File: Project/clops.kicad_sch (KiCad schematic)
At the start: 111 parts, among them IC1 W25Q16JVUXIQ, J1 USB_C_Receptacle_USB2.0, SW1 boot, SW2 RotaryEncoder_Switch, U2 USBLC6-2SC6, U3 RP2040, U4 XC6206PxxxMR-Regulator_Linear, Y1 12MHz

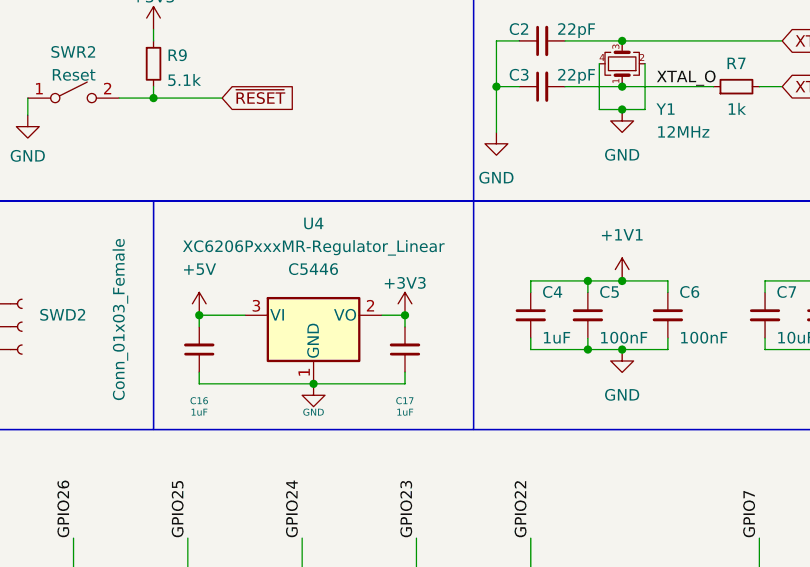
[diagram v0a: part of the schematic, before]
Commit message: Revert "update"
This reverts commit de9b7cebc370d770c1946fd24c0ccf0d0e181036.
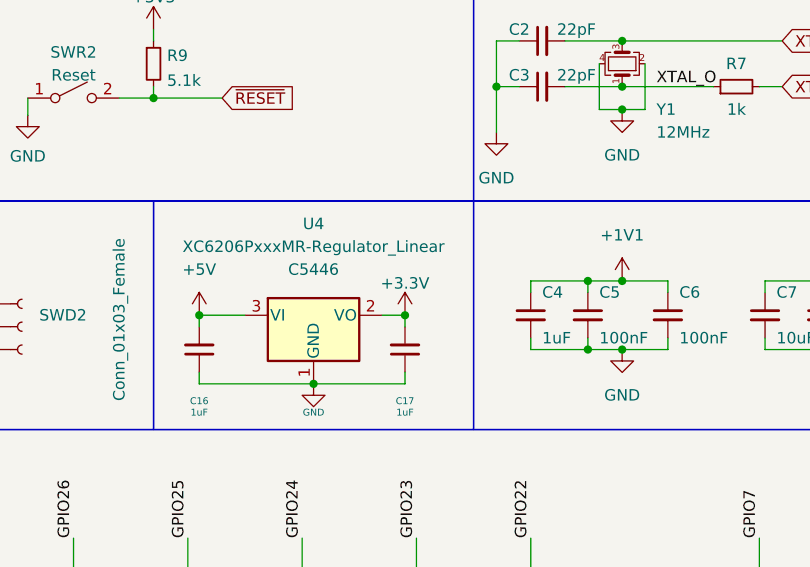
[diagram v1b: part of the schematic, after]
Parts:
- MX34: footprint PCM_marbastlib-mx:SW_MX_1u -> PCM_marbastlib-mx:SW_MX_HS_CPG151101S11_1u

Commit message: update
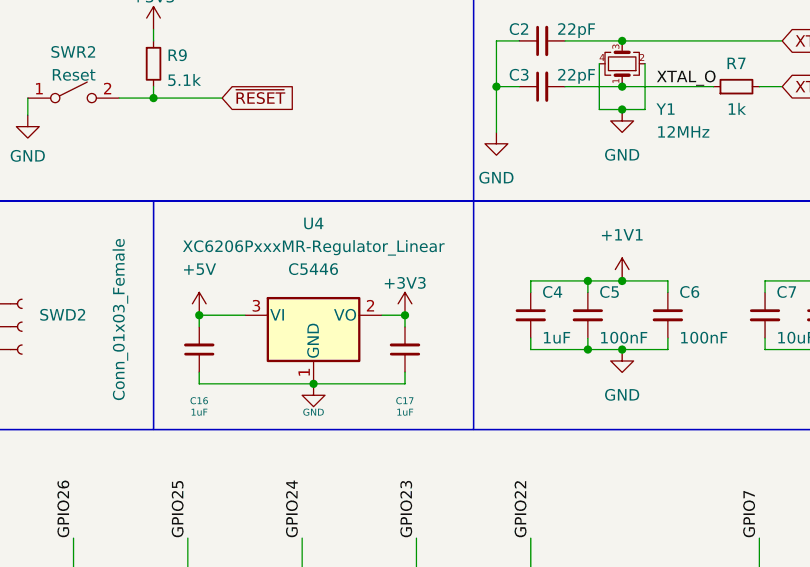
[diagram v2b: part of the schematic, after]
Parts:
- MX34: footprint PCM_marbastlib-mx:SW_MX_HS_CPG151101S11_1u -> PCM_marbastlib-mx:SW_MX_1u
